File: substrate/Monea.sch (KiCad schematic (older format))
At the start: 6 parts, among them J1 Conn_02x20_Odd_Even, J2 Conn_01x06_Female, J3 Conn_01x04_Female, J4 Conn_01x05_Female

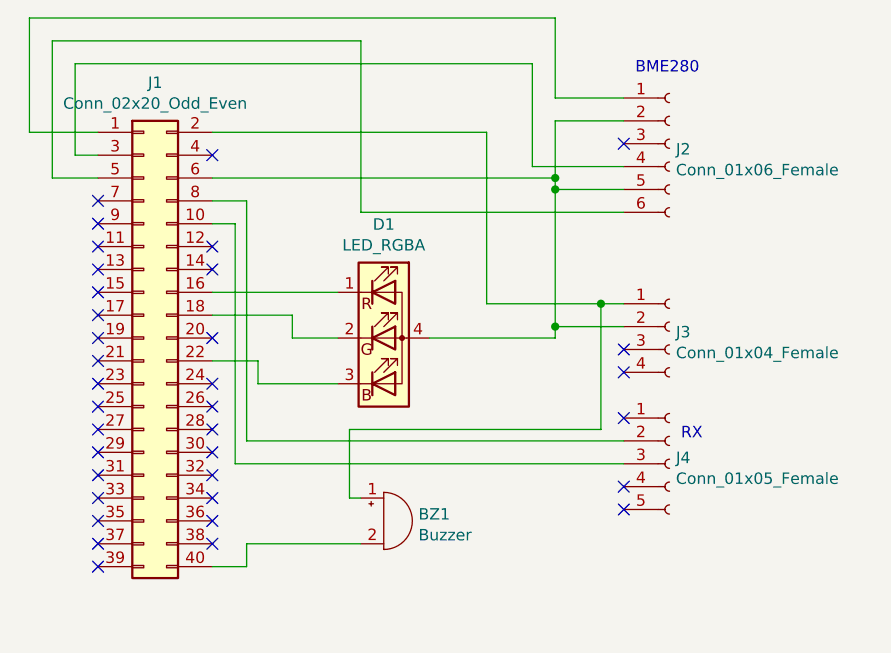
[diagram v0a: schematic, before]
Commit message: :construction: WIP
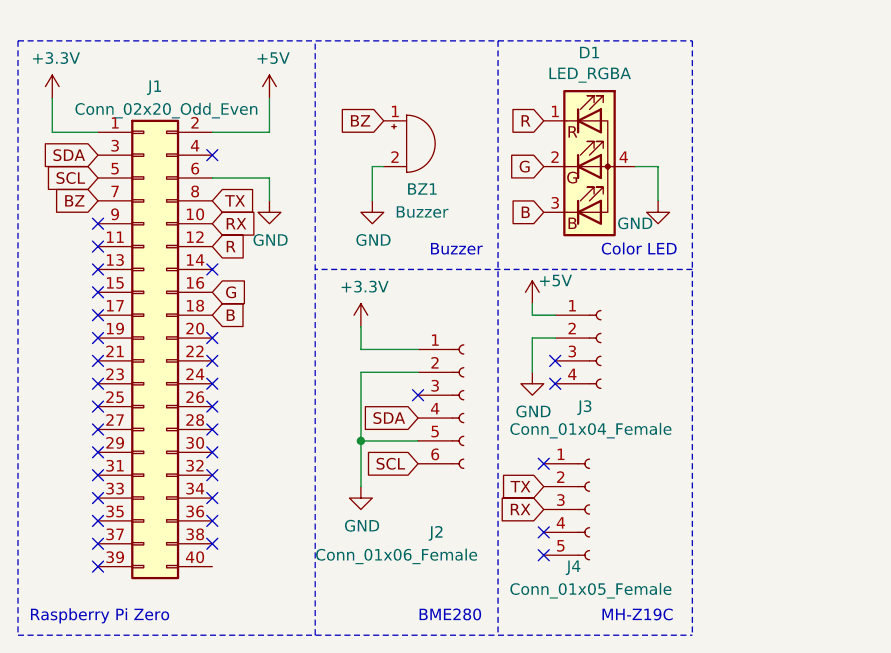
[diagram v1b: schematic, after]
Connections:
- net +3V3: now reaches J1.1 (Pin_1), J2.1 (Pin_1)
- net RX: now reaches J1.10 (Pin_10), J4.3 (Pin_3)
- net R: now reaches J1.12 (Pin_12)
- net R: now also D1.1 (RK)
- net G: now reaches J1.16 (Pin_16)
- net G: now also D1.2 (GK); no longer D1.1 (RK)
- net B: now reaches J1.18 (Pin_18)
- net B: now also D1.3 (BK); no longer D1.2 (GK)
- net +5V: now reaches J1.2 (Pin_2), J3.1 (Pin_1)
- net +5V: no longer BZ1.1 (-)
- net at J1.22 (Pin_22): no longer D1.3 (BK)
- net SDA: now reaches J1.3 (Pin_3), J2.4 (Pin_4)
- net at J1.40 (Pin_40): no longer BZ1.2 (+)
- net SCL: now reaches J1.5 (Pin_5), J2.6 (Pin_6)
- net GND: now reaches D1.4 (A), J1.6 (Pin_6), J2.2 (Pin_2), J2.5 (Pin_5), J3.2 (Pin_2)
- net GND: now also BZ1.2 (+)
- net BZ: now reaches J1.7 (Pin_7)
- net BZ: now also BZ1.1 (-)
- net TX: now reaches J1.8 (Pin_8), J4.2 (Pin_2)
- no-connect marks 35 -> 34
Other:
- note added: "Buzzer"
- note added: "Color LED"
- note added: "MH-Z19C"
- note added: "Raspberry Pi Zero"
- note removed: "RX"
- moved on the sheet: BZ1, D1, J2, J3, J4
